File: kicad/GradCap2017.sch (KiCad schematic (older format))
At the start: 20 parts

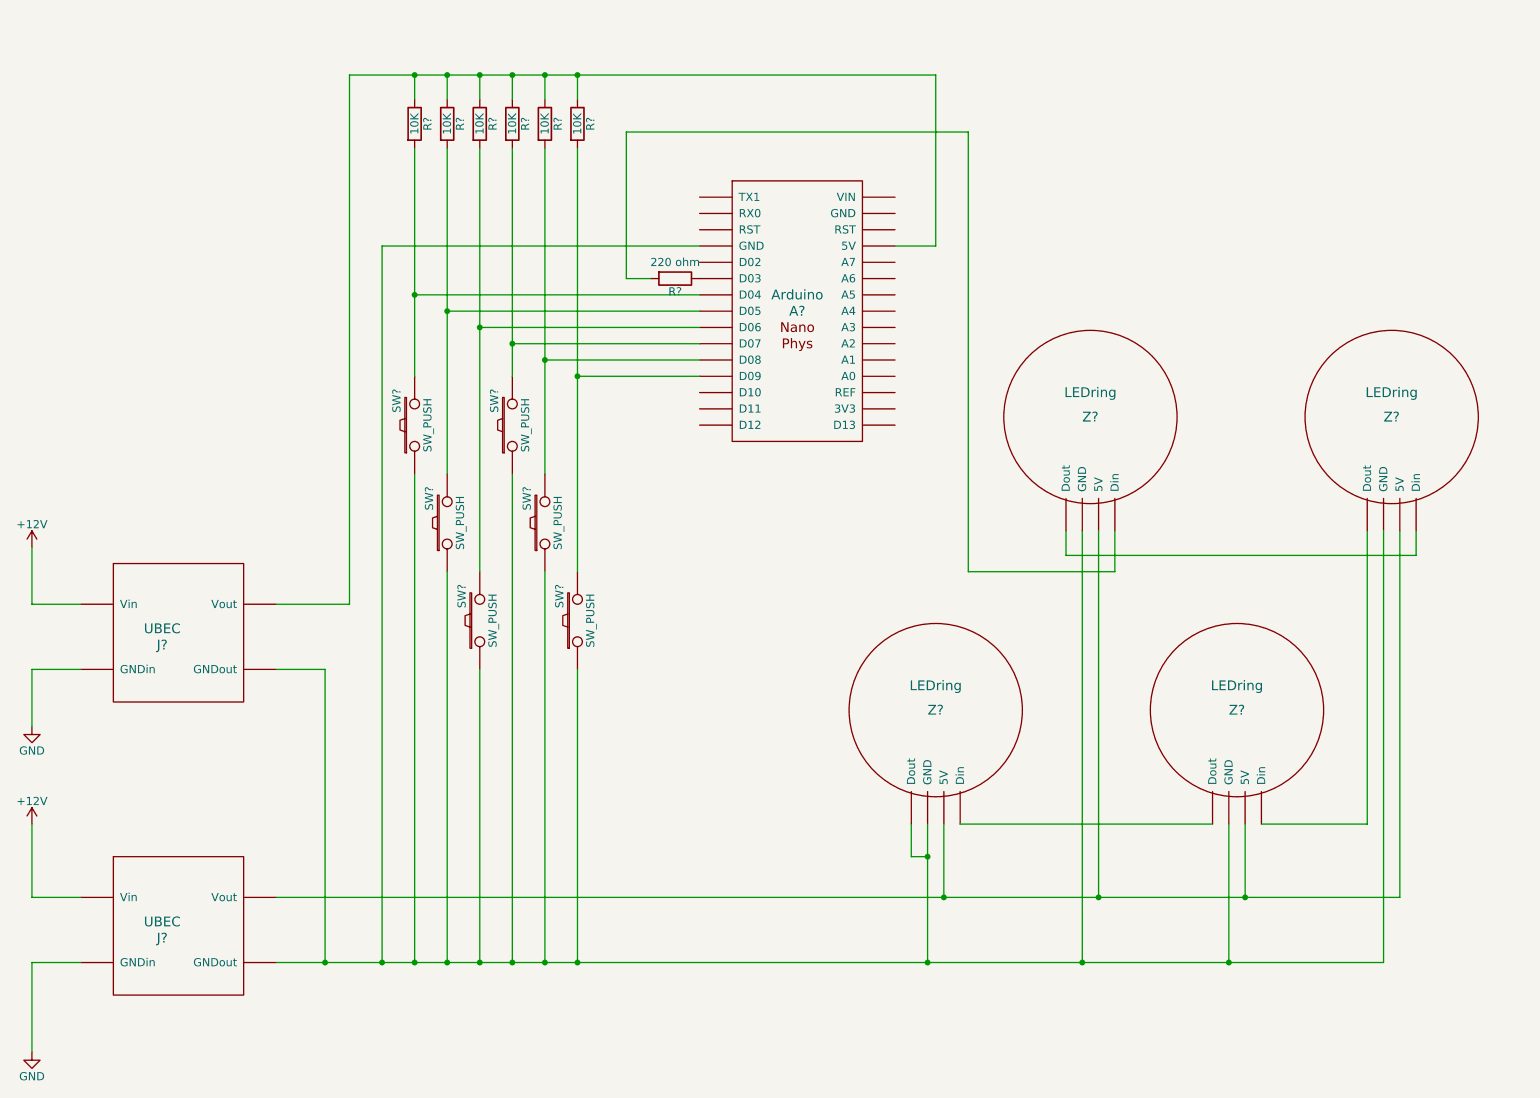
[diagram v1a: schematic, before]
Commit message: need four Arduinos
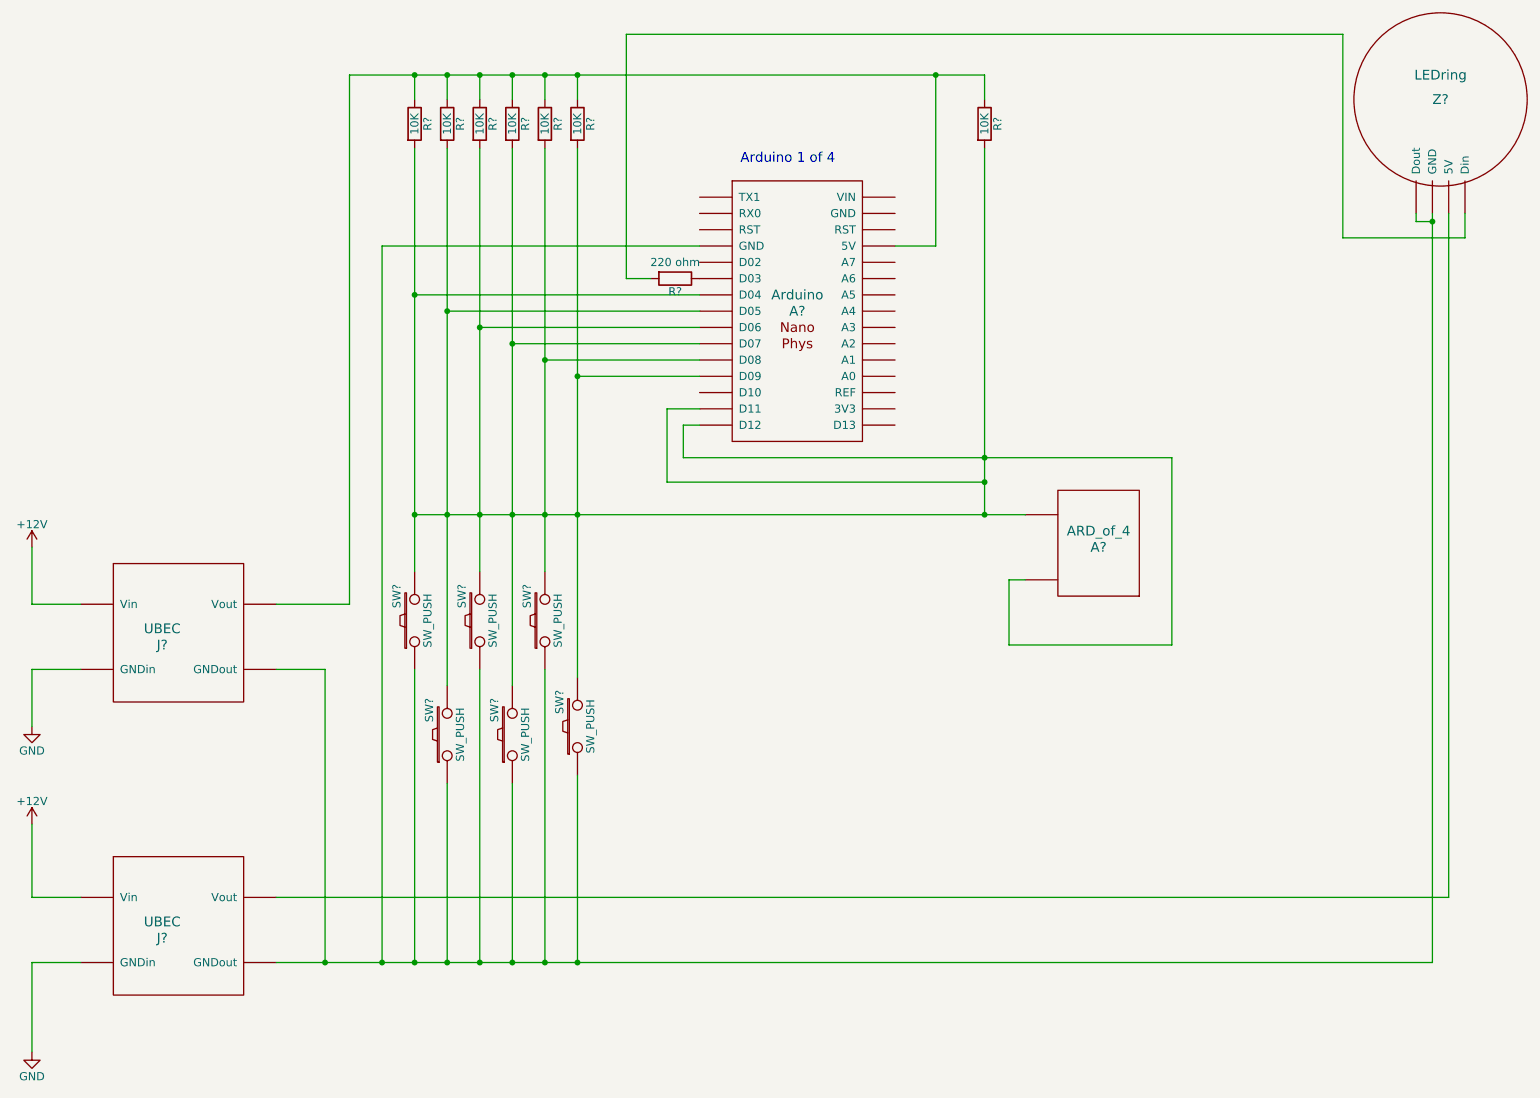
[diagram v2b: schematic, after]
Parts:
- removed Z? (x3): LEDring, symbol LEDring
- added A?: ARD_of_4, symbol ARD_of_4
- added R?: 10K, symbol R
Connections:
- net at Z?.~ (GND): now also J?.~ (Vout)
- net at A?.~ (VIN), J?.~ (Vout), R?.1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: now also R?.1
- net at A?.~ (VIN): now also R?.2, R?.2, R?.2, R?.2, R?.2, R?.2, SW?.2, SW?.2, SW?.2, SW?.2, SW?.2, SW?.2, A?.~ (output), R?.2
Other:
- note added: "Arduino 1 of 4"
- moved on the sheet: SW?, Z?
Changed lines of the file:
@@
 LIBS:switches
 LIBS:relays
+LIBS:motors
 LIBS:transistors
 LIBS:conn
@@
 LIBS:valves
 LIBS:mdoLibrary
+LIBS:Arduino_Nano-cache
 LIBS:GradCap2017-cache
 EELAYER 25 0
@@
 L LEDring Z?
 U 1 1 5A458774
-P 7750 3050
-F 0 "Z?" H 7750 3050 60  0000 C CNN
-F 1 "LEDring" H 7750 3200 60  0000 C CNN
-F 2 "" H 7750 3200 60  0001 C CNN
-F 3 "" H 7750 3200 60  0001 C CNN
-	1    7750 3050
-	1    0    0    -1
-$EndComp
-$Comp
-L LEDring Z?
-U 1 1 5A458E53
-P 9600 3050
-F 0 "Z?" H 9600 3050 60  0000 C CNN
-F 1 "LEDring" H 9600 3200 60  0000 C CNN
-F 2 "" H 9600 3200 60  0001 C CNN
-F 3 "" H 9600 3200 60  0001 C CNN
-	1    9600 3050
-	1    0    0    -1
-$EndComp
-$Comp
-L LEDring Z?
-U 1 1 5A458ECA
-P 6800 4850
-F 0 "Z?" H 6800 4850 60  0000 C CNN
-F 1 "LEDring" H 6800 5000 60  0000 C CNN
-F 2 "" H 6800 5000 60  0001 C CNN
-F 3 "" H 6800 5000 60  0001 C CNN
-	1    6800 4850
-	1    0    0    -1
-$EndComp
-$Comp
-L LEDring Z?
-U 1 1 5A458F51
-P 8650 4850
-F 0 "Z?" H 8650 4850 60  0000 C CNN
-F 1 "LEDring" H 8650 5000 60  0000 C CNN
-F 2 "" H 8650 5000 60  0001 C CNN
-F 3 "" H 8650 5000 60  0001 C CNN
-	1    8650 4850
+P 9900 1100
+F 0 "Z?" H 9900 1100 60  0000 C CNN
+F 1 "LEDring" H 9900 1250 60  0000 C CNN
+F 2 "" H 9900 1250 60  0001 C CNN
+F 3 "" H 9900 1250 60  0001 C CNN
+	1    9900 1100
 	1    0    0    -1
 $EndComp
@@
 	1    0    0    -1
 $EndComp
-Connection ~ 3050 6400
-Wire Wire Line
-	1250 6000 1250 5550
-Wire Wire Line
-	1550 6000 1250 6000
-Wire Wire Line
-	1250 6400 1250 6950
-Wire Wire Line
-	1550 6400 1250 6400
-Wire Wire Line
-	2750 6400 9550 6400
-Wire Wire Line
-	9450 3750 9450 5550
-Connection ~ 6750 5750
-Wire Wire Line
-	6650 5750 6750 5750
-Wire Wire Line
-	6650 5550 6650 5750
-Connection ~ 6850 6000
-Wire Wire Line
-	6850 5550 6850 6000
-Wire Wire Line
-	9550 6400 9550 3750
-Wire Wire Line
-	7700 3750 7700 6400
-Wire Wire Line
-	8700 6000 8700 5550
-Wire Wire Line
-	8600 6400 8600 5550
-Wire Wire Line
-	6750 5550 6750 6400
-Connection ~ 6750 6400
-Wire Wire Line
-	7800 6000 7800 3750
-Wire Wire Line
-	9650 6000 9650 3750
-Wire Wire Line
-	2750 6000 9650 6000
-Wire Wire Line
-	7900 4000 7900 3750
-Wire Wire Line
-	8500 5550 6950 5550
-Wire Wire Line
-	9450 5550 8800 5550
-Wire Wire Line
-	9750 3900 9750 3750
-Wire Wire Line
-	7600 3750 7600 3900
-Wire Wire Line
-	3050 4600 3050 6400
-Wire Wire Line
-	2750 4600 3050 4600
-Wire Wire Line
-	1250 4200 1550 4200
-Wire Wire Line
-	1250 3850 1250 4200
-Wire Wire Line
-	1250 4600 1550 4600
-Wire Wire Line
-	1250 4950 1250 4600
-Wire Wire Line
-	7600 3900 9750 3900
-Connection ~ 7700 6400
-Connection ~ 8600 6400
-Connection ~ 8700 6000
-Connection ~ 7800 6000
 $Comp
 L Arduino A?
@@
 	1    0    0    -1
 $EndComp
-Wire Wire Line
-	7000 4000 7900 4000
-Wire Wire Line
-	3200 4200 2750 4200
-Wire Wire Line
-	3200 950  3200 4200
-Connection ~ 3400 6400
-Wire Wire Line
-	3400 6400 3400 2000
-Wire Wire Line
-	3400 2000 5350 2000
-Wire Wire Line
-	5050 2200 4900 2200
-Wire Wire Line
-	4900 2200 4900 1300
-Wire Wire Line
-	4900 1300 7000 1300
-Wire Wire Line
-	7000 1300 7000 4000
-Wire Wire Line
-	3200 950  6800 950
-Wire Wire Line
-	6800 950  6800 2000
-Wire Wire Line
-	6800 2000 6550 2000
 $Comp
 L SW_PUSH SW?
 U 1 1 5A4908F2
-P 3600 3100
-F 0 "SW?" H 3750 3210 50  0000 C CNN
-F 1 "SW_PUSH" H 3600 3020 50  0000 C CNN
-F 2 "" H 3600 3100 60  0000 C CNN
-F 3 "" H 3600 3100 60  0000 C CNN
-	1    3600 3100
+P 3600 4300
+F 0 "SW?" H 3750 4410 50  0000 C CNN
+F 1 "SW_PUSH" H 3600 4220 50  0000 C CNN
+F 2 "" H 3600 4300 60  0000 C CNN
+F 3 "" H 3600 4300 60  0000 C CNN
+	1    3600 4300
 	0    -1   -1   0
 $EndComp
@@
 L SW_PUSH SW?
 U 1 1 5A490A65
-P 3800 3700
-F 0 "SW?" H 3950 3810 50  0000 C CNN
-F 1 "SW_PUSH" H 3800 3620 50  0000 C CNN
-F 2 "" H 3800 3700 60  0000 C CNN
-F 3 "" H 3800 3700 60  0000 C CNN
-	1    3800 3700
+P 3800 5000
+F 0 "SW?" H 3950 5110 50  0000 C CNN
+F 1 "SW_PUSH" H 3800 4920 50  0000 C CNN
+F 2 "" H 3800 5000 60  0000 C CNN
+F 3 "" H 3800 5000 60  0000 C CNN
+	1    3800 5000
 	0    -1   -1   0
 $EndComp
@@
 L SW_PUSH SW?
 U 1 1 5A490D81
-P 4200 3100
-F 0 "SW?" H 4350 3210 50  0000 C CNN
-F 1 "SW_PUSH" H 4200 3020 50  0000 C CNN
-F 2 "" H 4200 3100 60  0000 C CNN
-F 3 "" H 4200 3100 60  0000 C CNN
-	1    4200 3100
+P 4200 5000
+F 0 "SW?" H 4350 5110 50  0000 C CNN
+F 1 "SW_PUSH" H 4200 4920 50  0000 C CNN
+F 2 "" H 4200 5000 60  0000 C CNN
+F 3 "" H 4200 5000 60  0000 C CNN
+	1    4200 5000
 	0    -1   -1   0
 $EndComp
@@
 L SW_PUSH SW?
 U 1 1 5A490DC1
-P 4400 3700
-F 0 "SW?" H 4550 3810 50  0000 C CNN
-F 1 "SW_PUSH" H 4400 3620 50  0000 C CNN
-F 2 "" H 4400 3700 60  0000 C CNN
-F 3 "" H 4400 3700 60  0000 C CNN
-	1    4400 3700
+P 4400 4300
+F 0 "SW?" H 4550 4410 50  0000 C CNN
+F 1 "SW_PUSH" H 4400 4220 50  0000 C CNN
+F 2 "" H 4400 4300 60  0000 C CNN
+F 3 "" H 4400 4300 60  0000 C CNN
+	1    4400 4300
 	0    -1   -1   0
 $EndComp
@@
 L SW_PUSH SW?
 U 1 1 5A490E07
-P 4600 4300
-F 0 "SW?" H 4750 4410 50  0000 C CNN
-F 1 "SW_PUSH" H 4600 4220 50  0000 C CNN
-F 2 "" H 4600 4300 60  0000 C CNN
-F 3 "" H 4600 4300 60  0000 C CNN
-	1    4600 4300
-	0    -1   -1   0
-$EndComp
-Wire Wire Line
-	5350 2300 3600 2300
-Wire Wire Line
-	3600 1400 3600 2800
-Wire Wire Line
-	5350 2400 3800 2400
-Wire Wire Line
-	3800 1400 3800 3400
-Wire Wire Line
-	5350 2500 4000 2500
-Wire Wire Line
-	4000 1400 4000 4000
-Wire Wire Line
-	5350 2600 4200 2600
-Wire Wire Line
-	4200 1400 4200 2800
-Wire Wire Line
-	5350 2700 4400 2700
-Wire Wire Line
-	4400 1400 4400 3400
-Wire Wire Line
-	5350 2800 4600 2800
-Wire Wire Line
-	4600 1400 4600 4000
-Wire Wire Line
-	3600 3400 3600 6400
-Connection ~ 3600 6400
-Wire Wire Line
-	3800 4000 3800 6400
-Connection ~ 3800 6400
-Wire Wire Line
-	4000 4600 4000 6400
-Connection ~ 4000 6400
-Wire Wire Line
-	4200 3400 4200 6400
-Connection ~ 4200 6400
-Wire Wire Line
-	4400 4000 4400 6400
-Connection ~ 4400 6400
-Wire Wire Line
-	4600 4600 4600 6400
-Connection ~ 4600 6400
+P 4600 4950
+F 0 "SW?" H 4750 5060 50  0000 C CNN
+F 1 "SW_PUSH" H 4600 4870 50  0000 C CNN
+F 2 "" H 4600 4950 60  0000 C CNN
+F 3 "" H 4600 4950 60  0000 C CNN
+	1    4600 4950
+	0    -1   -1   0
+$EndComp
 $Comp
 L R R?
@@
 	1    0    0    -1
 $EndComp
+Text Notes 5600 1500 0    60   ~ 0
+Arduino 1 of 4
+$Comp
+L R R?
+U 1 1 5A767559
+P 7100 1250
+F 0 "R?" V 7180 1250 50  0000 C CNN
+F 1 "10K" V 7100 1250 50  0000 C CNN
+F 2 "" V 7030 1250 30  0000 C CNN
+F 3 "" H 7100 1250 30  0000 C CNN
+	1    7100 1250
+	1    0    0    -1
+$EndComp
+$Comp
+L ARD_of_4 A?
+U 1 1 5A7681AD
+P 7800 3850
+F 0 "A?" H 7800 3850 60  0000 C CNN
+F 1 "ARD_of_4" H 7800 3950 60  0000 C CNN
+F 2 "" H 7800 3850 60  0001 C CNN
+F 3 "" H 7800 3850 60  0001 C CNN
+	1    7800 3850
+	1    0    0    -1
+$EndComp
+Connection ~ 3050 6400
+Wire Wire Line
+	1250 6000 1250 5550
+Wire Wire Line
+	1550 6000 1250 6000
+Wire Wire Line
+	1250 6400 1250 6950
+Wire Wire Line
+	1550 6400 1250 6400
+Wire Wire Line
+	9850 6400 2750 6400
+Wire Wire Line
+	9850 1800 9850 6400
+Wire Wire Line
+	3050 4600 3050 6400
+Wire Wire Line
+	2750 4600 3050 4600
+Wire Wire Line
+	1250 4200 1550 4200
+Wire Wire Line
+	1250 3850 1250 4200
+Wire Wire Line
+	1250 4600 1550 4600
+Wire Wire Line
+	1250 4950 1250 4600
+Wire Wire Line
+	3200 4200 2750 4200
+Wire Wire Line
+	3200 950  3200 4200
+Connection ~ 3400 6400
+Wire Wire Line
+	3400 6400 3400 2000
+Wire Wire Line
+	3400 2000 5350 2000
+Wire Wire Line
+	5050 2200 4900 2200
+Wire Wire Line
+	4900 2200 4900 700
+Wire Wire Line
+	4900 700  9300 700
+Wire Wire Line
+	3200 950  7100 950
+Wire Wire Line
+	6800 950  6800 2000
+Wire Wire Line
+	6800 2000 6550 2000
+Wire Wire Line
+	5350 2300 3600 2300
+Wire Wire Line
+	3600 1400 3600 4000
+Wire Wire Line
+	5350 2400 3800 2400
+Wire Wire Line
+	3800 1400 3800 4700
+Wire Wire Line
+	5350 2500 4000 2500
+Wire Wire Line
+	4000 1400 4000 4000
+Wire Wire Line
+	5350 2600 4200 2600
+Wire Wire Line
+	4200 1400 4200 4700
+Wire Wire Line
+	5350 2700 4400 2700
+Wire Wire Line
+	4400 1400 4400 4000
+Wire Wire Line
+	5350 2800 4600 2800
+Wire Wire Line
+	4600 1400 4600 4650
+Wire Wire Line
+	3600 4600 3600 6400
+Connection ~ 3600 6400
+Wire Wire Line
+	3800 5300 3800 6400
+Connection ~ 3800 6400
+Wire Wire Line
+	4000 4600 4000 6400
+Connection ~ 4000 6400
+Wire Wire Line
+	4200 5300 4200 6400
+Connection ~ 4200 6400
+Wire Wire Line
+	4400 4600 4400 6400
+Connection ~ 4400 6400
+Wire Wire Line
+	4600 6400 4600 5250
+Connection ~ 4600 6400
 Wire Wire Line
 	3600 1100 3600 950
@@
 Connection ~ 4400 2700
 Connection ~ 4600 2800
+Wire Wire Line
+	2750 6000 9950 6000
+Wire Wire Line
+	9950 6000 9950 1800
+Wire Wire Line
+	9300 700  9300 1950
+Wire Wire Line
+	9300 1950 10050 1950
+Wire Wire Line
+	10050 1950 10050 1800
+Wire Wire Line
+	9750 1800 9750 1850
+Wire Wire Line
+	9750 1850 9850 1850
+Connection ~ 9850 1850
+Wire Wire Line
+	7100 950  7100 1100
+Connection ~ 6800 950
+Wire Wire Line
+	3600 3650 7350 3650
+Connection ~ 4600 3650
+Connection ~ 4400 3650
+Connection ~ 4200 3650
+Connection ~ 4000 3650
+Connection ~ 3800 3650
+Connection ~ 3600 3650
+Wire Wire Line
+	7100 1400 7100 3650
+Connection ~ 7100 3650
+Wire Wire Line
+	5350 3100 5250 3100
+Wire Wire Line
+	5250 3100 5250 3300
+Wire Wire Line
+	5250 3300 8250 3300
+Connection ~ 7100 3300
+Wire Wire Line
+	7350 4050 7250 4050
+Wire Wire Line
+	7250 4050 7250 4450
+Wire Wire Line
+	7250 4450 8250 4450
+Wire Wire Line
+	8250 4450 8250 3300
+Wire Wire Line
+	5350 3000 5150 3000
+Wire Wire Line
+	5150 3000 5150 3450
+Wire Wire Line
+	5150 3450 7100 3450
+Connection ~ 7100 3450
 $EndSCHEMATC
